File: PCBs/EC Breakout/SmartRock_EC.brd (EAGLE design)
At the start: 80.3 x 37.3 mm, 53 parts, among them IC2 TL074P, U1 ADS1115IDGST, U2 TPS60400DBVR

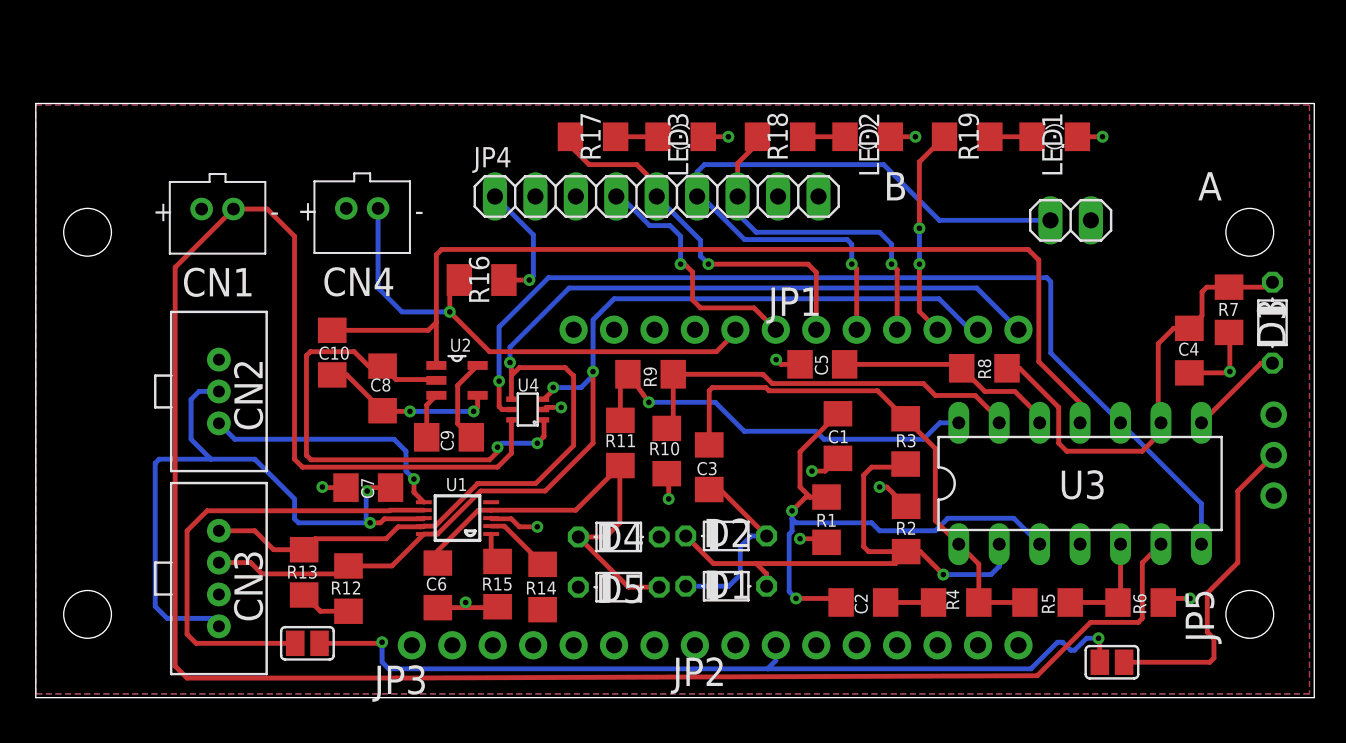
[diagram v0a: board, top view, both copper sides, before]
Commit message: Breakout Board Fix
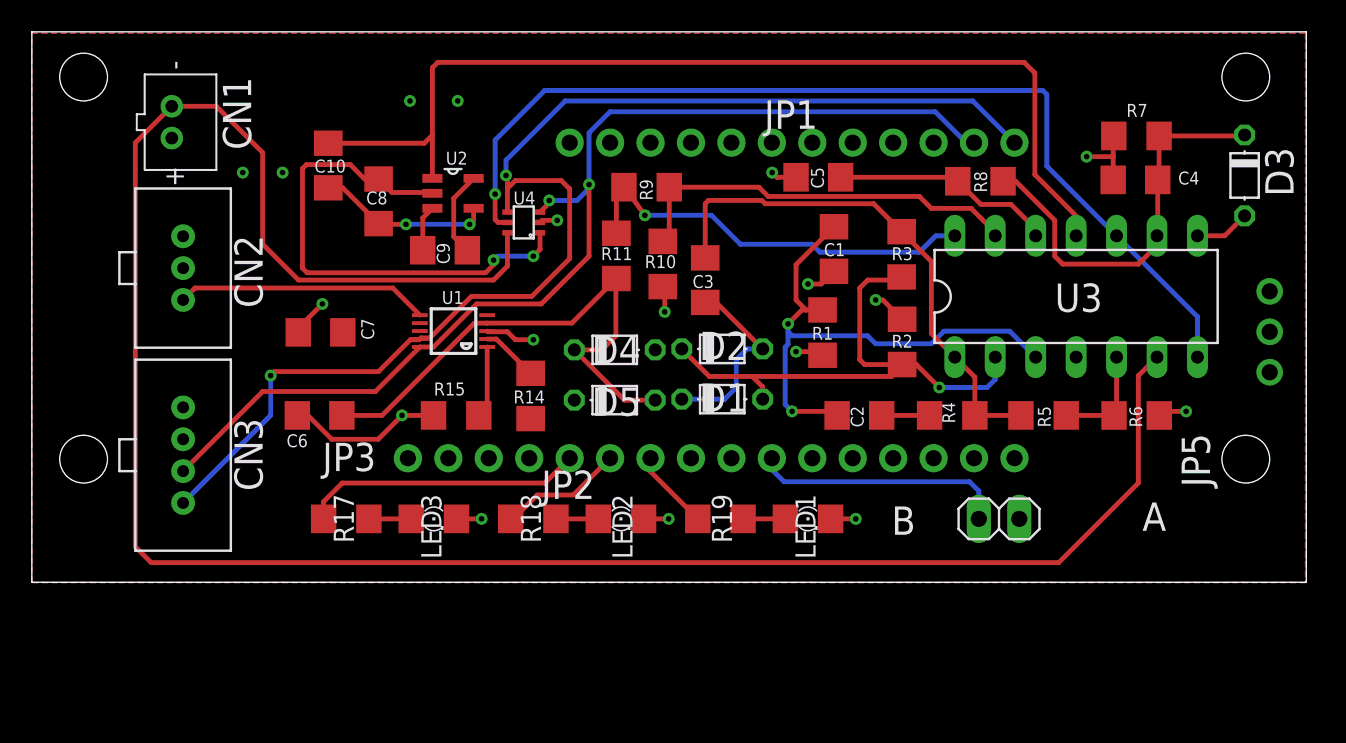
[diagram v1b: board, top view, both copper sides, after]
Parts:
- removed CN4: (no value), adafruit:JST-PH-2-THM
- removed JP4: (no value), pinhead:1X09
- removed R12, R13: 10k, rcl:R1206
- removed R16: (no value), adafruit:M1206
- removed SJ1, SJ2: (no value), jumper:SJ
- R17, R18, R19: value 10k -> 3.3k
- moved LED1 28.6 mm to (60.5, 12.2)
- moved LED2 28.6 mm to (48.8, 12.2)
- moved LED3 28.6 mm to (37.0, 12.2)
- moved R17 28.6 mm to (31.5, 12.2)
- moved R18 28.6 mm to (43.2, 12.2)
- moved R19 28.6 mm to (55.0, 12.2)
- moved REED 19.3 mm to (72.5, 12.2)
- moved C6 13.0 mm to (29.8, 18.7), turned to 0 degrees
- moved R7 12.4 mm to (81.1, 36.3), turned to 0 degrees
- moved R14 12.0 mm to (43.1, 20.0)
- moved JP1 11.8 mm to (59.5, 35.9)
- moved U2 11.8 mm to (38.2, 32.7)
- moved R1 11.8 mm to (61.4, 23.9)
- moved U1 11.8 mm to (38.2, 24.0)
- moved C1 11.8 mm to (62.1, 29.2)
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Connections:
- removed net 3VO: JP4.2
- removed net FLT: JP4.8
- removed net INT: CN4.2, JP1.8, R16.1
- removed net N$6: JP5.2, SJ2.2
- removed net RDY: JP4.9
- net AIN3: no longer SJ1.1
- net GND: now also U$7.P$3; no longer CN4.1, JP4.3, U$7.P$2
- net GPIO10: no longer JP4.5, R17.1
- net GPIO11: no longer JP4.4
- net GPIO5: no longer R19.1
- net GPIO6: no longer JP4.7, R18.1
- net GPIO9: no longer JP4.6, REED.1
- net GPIOA0: now also R17.1
- net GPIOA1: now also R18.1
- net GPIOA2: now also R19.1
- net GPIOA5: now also REED.1; no longer SJ1.2, SJ2.1
- net SCL: now also U$7.P$2; no longer R12.2, U$7.P$3
- net SDA: now also U$7.P$1; no longer R13.2, U$7.P$4
- net VCC: now also U$7.P$4; no longer JP4.1, R12.1, R13.1, R16.2, U$7.P$1
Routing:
- net VCC: track 86.2 -> 32.1 mm, vias 5 -> 6
- net GPIO9: track 41.8 -> 0.00 mm, vias 1 -> 0
- net GPIOA5: track 54.8 -> 16.0 mm, vias 2 -> 0
- net INT: track 32.0 -> 0.00 mm, vias 1 -> 0
- net AIN3: track 28.9 -> 0.00 mm
- net GPIO10: track 23.9 -> 0.00 mm, vias 1 -> 0
- net GPIO6: track 21.3 -> 0.00 mm, vias 1 -> 0
- net N$6: track 20.4 -> 0.00 mm
- net GPIOA0: track 0.00 -> 17.7 mm
- net GPIO11: track 15.5 -> 0.00 mm, vias 1 -> 0
- net GPIO5: track 13.2 -> 0.00 mm, vias 2 -> 0
- net GPIOA1: track 0.00 -> 8.06 mm
- net SDA: track 72.1 -> 78.7 mm, vias 1 -> 2
- net AOUT: track 27.4 -> 33.8 mm
- net GND: track 41.5 -> 47.6 mm
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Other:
- board size 80.3 x 37.3 mm -> 80 x 34.6 mm
- board text removed: "CN4"
- board text removed: "R12"
- board text removed: "R13"

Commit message: Updated Board and Code
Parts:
- R17: value 3.3k -> 1k
- R18, R19: value 3.3k -> 4.7k
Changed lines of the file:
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@@
 <element name="U$7" library="JSTconnector" package="JST_4PIN_2MM" value="JST_4PIN_2MM" x="21.25" y="13.25" smashed="yes" rot="R270"/>
 <element name="U$9" library="JSTconnector" package="JST_3PIN_2MM" value="JST_3PIN_2MM" x="21.25" y="28" smashed="yes" rot="R270"/>
-<element name="R17" library="rcl" library_urn="urn:adsk.eagle:library:334" package="R1206" package3d_urn="urn:adsk.eagle:package:23540/2" value="3.3k" x="31.5" y="12.25" smashed="yes">
+<element name="R17" library="rcl" library_urn="urn:adsk.eagle:library:334" package="R1206" package3d_urn="urn:adsk.eagle:package:23540/2" value="1k" x="31.5" y="12.25" smashed="yes">
 <attribute name="NAME" x="31.98" y="10.73" size="1.27" layer="25" rot="R90"/>
 <attribute name="POPULARITY" value="19" x="31.5" y="12.25" size="1.778" layer="27" display="off"/>
 <attribute name="SPICEPREFIX" value="R" x="31.5" y="12.25" size="1.778" layer="27" display="off"/>
 </element>
-<element name="R18" library="rcl" library_urn="urn:adsk.eagle:library:334" package="R1206" package3d_urn="urn:adsk.eagle:package:23540/2" value="3.3k" x="43.25" y="12.25" smashed="yes">
+<element name="R18" library="rcl" library_urn="urn:adsk.eagle:library:334" package="R1206" package3d_urn="urn:adsk.eagle:package:23540/2" value="4.7k" x="43.25" y="12.25" smashed="yes">
 <attribute name="NAME" x="43.73" y="10.73" size="1.27" layer="25" rot="R90"/>
 <attribute name="POPULARITY" value="19" x="43.25" y="12.25" size="1.778" layer="27" display="off"/>
 <attribute name="SPICEPREFIX" value="R" x="43.25" y="12.25" size="1.778" layer="27" display="off"/>
 </element>
-<element name="R19" library="rcl" library_urn="urn:adsk.eagle:library:334" package="R1206" package3d_urn="urn:adsk.eagle:package:23540/2" value="3.3k" x="55" y="12.25" smashed="yes">
+<element name="R19" library="rcl" library_urn="urn:adsk.eagle:library:334" package="R1206" package3d_urn="urn:adsk.eagle:package:23540/2" value="4.7k" x="55" y="12.25" smashed="yes">
 <attribute name="NAME" x="55.73" y="10.73" size="1.27" layer="25" rot="R90"/>
 <attribute name="POPULARITY" value="19" x="55" y="12.25" size="1.778" layer="27" display="off"/>
